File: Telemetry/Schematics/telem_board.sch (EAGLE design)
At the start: 29 parts, among them IC1 PIC18F26K80I/SP, IC2 PTN78000WAH, IC3 ISO1050DUB, IC4 SN75LBC179D, J1 ICD, J2 CANBUS, J3 CANBUS, J4 HALLSENS, J5 TEMPSENS, J7 RADIO, Q4 20M, X1 +12V

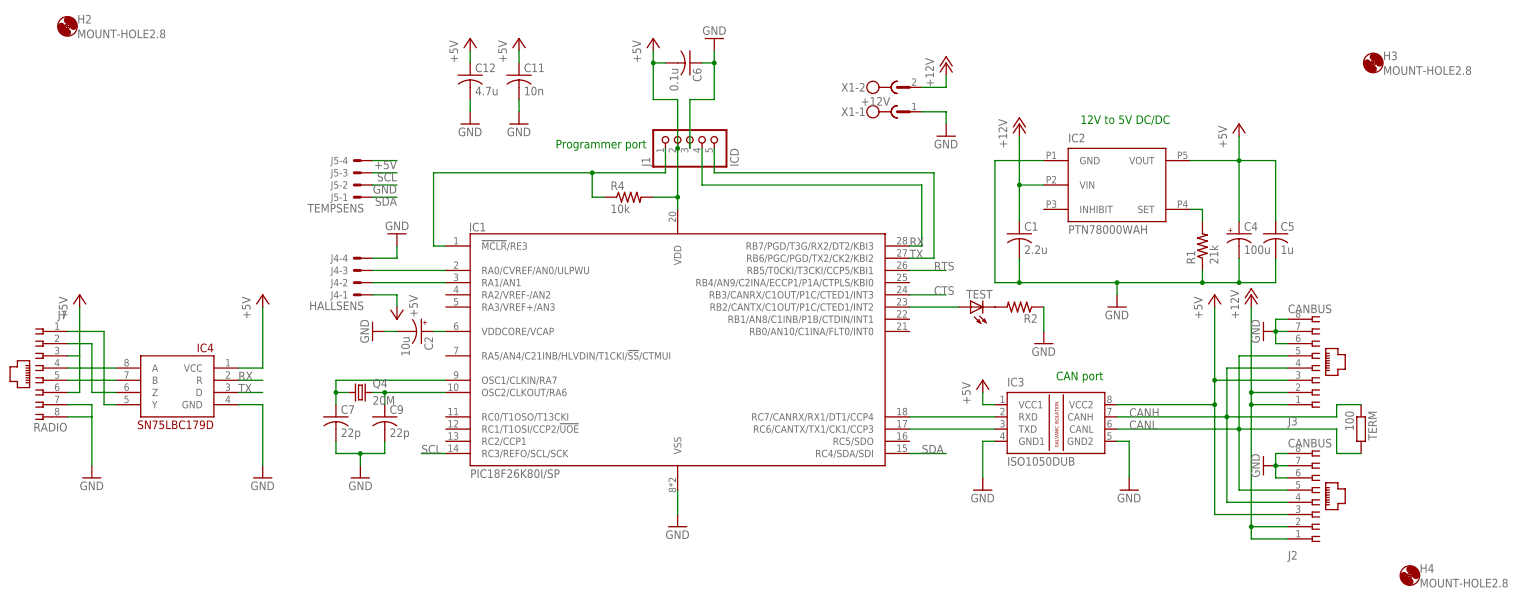
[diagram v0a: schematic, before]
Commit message: telem_board_v6
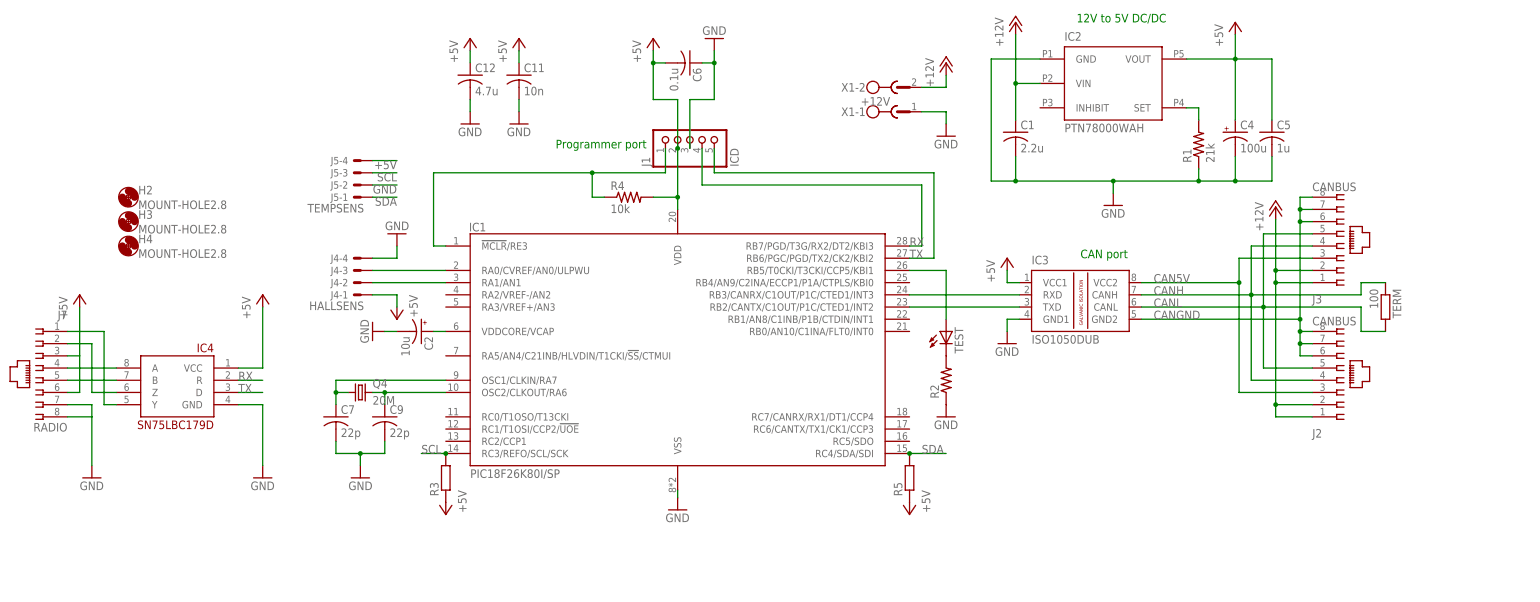
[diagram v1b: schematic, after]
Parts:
- added R3, R5: (no value), eagle-ltspice:R
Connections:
- removed net CTS: IC1.RB3/CANRX/C1OUT/P1C/CTED1/INT3
- removed net N$18: IC1.RC7/CANRX/RX1/DT1/CCP4, IC3.RXD
- removed net RTS: IC1.RB5/T0CKI/T3CKI/CCP5/KBI1
- new net CAN5V: IC3.VCC2, J2.3, J3.3
- new net CANGND: IC3.GND2, J2.6, J2.7, J2.8, J3.6, J3.7, J3.8
- new net N$9: IC1.RB3/CANRX/C1OUT/P1C/CTED1/INT3, IC3.RXD
- net +5V: now also R3.1, R5.1; no longer IC3.VCC2, J2.3, J3.3
- net GND: no longer IC3.GND2, J2.6, J2.7, J2.8, J3.6, J3.7, J3.8
- net N$11: now also IC1.RB5/T0CKI/T3CKI/CCP5/KBI1, TEST.A; no longer IC1.RC6/CANTX/TX1/CK1/CCP3, IC3.TXD
- net N$6: now also IC3.TXD; no longer TEST.A
- net SCL: now also R3.2
- net SDA: now also R5.2
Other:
- moved on the sheet: C1, C4, C5, H2, H3, H4, IC2, IC3, J2, J3, R1, R2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
